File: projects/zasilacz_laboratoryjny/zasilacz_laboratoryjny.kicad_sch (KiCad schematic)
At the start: 99 parts, among them J1 OUT+, J10 PWRL−, J100 BARREL JACK, J101 BANANA JACK, J102 BANANA JACK, J103 OFF_BOARD, J104 OFF_BOARD, J105 OFF_BOARD, J106 OFF_BOARD, J107 OFF_BOARD, J108 OFF_BOARD, J109 OFF_BOARD, J11 VSET1, J110 OFF_BOARD, J111 OFF_BOARD, J112 OFF_BOARD, J113 OFF_BOARD, J114 OFF_BOARD, J115 OFF_BOARD, J116 OFF_BOARD, J117 OFF_BOARD, J118 OFF_BOARD, J119 OFF_BOARD, J12 VSET2, J120 OFF_BOARD, J121 OFF_BOARD, J122 OFF_BOARD, J13 OCPL+, J14 OCPL−, J15 VDOL+, J16 VDOL−, J17 OCP1, J18 OCP2, J19 OCP3, J2 OUT-, J20 OCP4, J21 OCP5, J22 OCP6, J23 OCP7, J24 OCP8, J3 PWRIN, J4 PWRSW, J5 VMPROBE, J6 VMPWR, J7 VMGND, J8 OCP0, J9 PWRL+, M1 DIGITAL_VM, P1 10kΩ, SW1 SW_SP8T, SW2 SW_SPST, T1 BC557, T2 BC557, T3 BC547, T4 BC547, T5 BC557, T6 BC557, T7 BC517, T8 BC547, U1 DB207, U2 LM317, Y1 3V

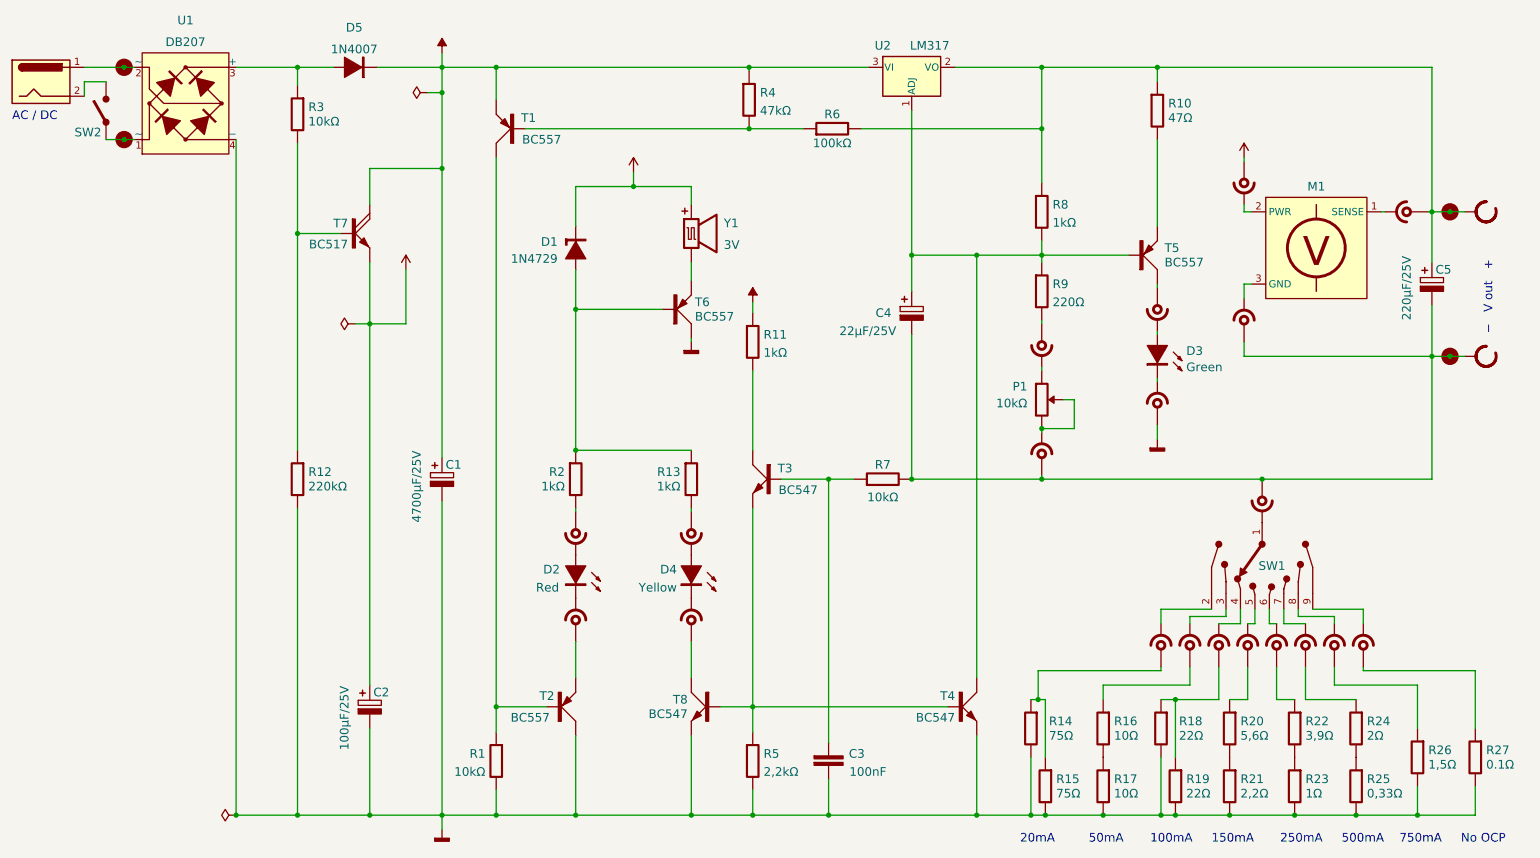
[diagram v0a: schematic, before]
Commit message: Zasilacz laboratoryjny - koniec
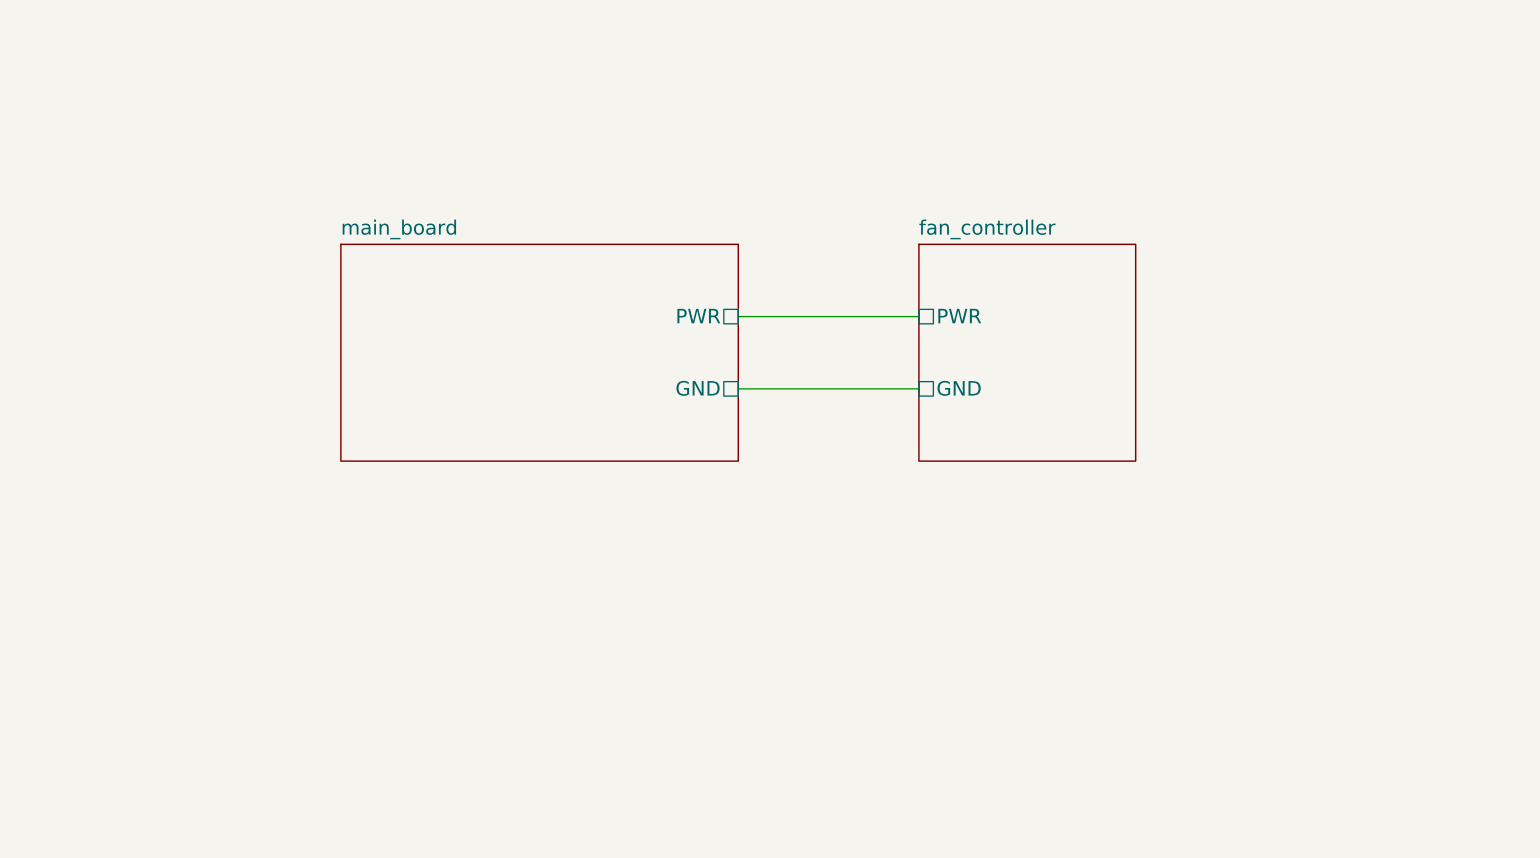
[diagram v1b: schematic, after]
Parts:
- removed C1: 4700μF/25V, VeeCad:RA3_6, symbol *Custom_Generic:C_Polarized
- removed C2: 100μF/25V, VeeCad:RA1_2, symbol *Custom_Generic:C_Polarized
- removed C3: 100nF, VeeCad:AX1_1N, symbol *Custom_Generic:C
- removed C4: 22μF/25V, VeeCad:RA1_2, symbol *Custom_Generic:C_Polarized
- removed C5: 220μF/25V, VeeCad:RA1_3, symbol *Custom_Generic:C_Polarized
- removed D1: 1N4729, VeeCad:AX2_1, symbol *Custom_Generic:D_zener
- removed D2: Red, symbol *Custom_Generic:LED
- removed D3: Green, symbol *Custom_Generic:LED
- removed D4: Yellow, symbol *Custom_Generic:LED
- removed D5: 1N4007, VeeCad:VERTAX_1U, symbol *Custom_Generic:D
- removed J1: OUT+, VeeCad:WIREPOINT, symbol *Custom_Generic:Wire_Solderpoint
- removed J10: PWRL−, VeeCad:SIP1, symbol *Custom_Generic:Conn_Point_M
- removed J100: BARREL JACK, symbol Connector:Barrel_Jack
- removed J101, J102: BANANA JACK, symbol *Custom_Generic:Conn_Jack
- removed J103, J104, J105, J106, J107, J108, J109, J110, J111, J112, J113, J114, J115, J116, J117, J118, J119, J120, J121, J122: OFF_BOARD, symbol *Custom_Generic:Conn_Point_F
- removed J11: VSET1, VeeCad:SIP1, symbol *Custom_Generic:Conn_Point_M
- removed J12: VSET2, VeeCad:SIP1, symbol *Custom_Generic:Conn_Point_M
- removed J13: OCPL+, VeeCad:SIP1, symbol *Custom_Generic:Conn_Point_M
- removed J14: OCPL−, VeeCad:SIP1, symbol *Custom_Generic:Conn_Point_M
- removed J15: VDOL+, VeeCad:SIP1, symbol *Custom_Generic:Conn_Point_M
- removed J16: VDOL−, VeeCad:SIP1, symbol *Custom_Generic:Conn_Point_M
- removed J17: OCP1, VeeCad:SIP1, symbol *Custom_Generic:Conn_Point_M
- removed J18: OCP2, VeeCad:SIP1, symbol *Custom_Generic:Conn_Point_M
- removed J19: OCP3, VeeCad:SIP1, symbol *Custom_Generic:Conn_Point_M
- removed J2: OUT-, VeeCad:WIREPOINT, symbol *Custom_Generic:Wire_Solderpoint
- removed J20: OCP4, VeeCad:SIP1, symbol *Custom_Generic:Conn_Point_M
- removed J21: OCP5, VeeCad:SIP1, symbol *Custom_Generic:Conn_Point_M
- removed J22: OCP6, VeeCad:SIP1, symbol *Custom_Generic:Conn_Point_M
- removed J23: OCP7, VeeCad:SIP1, symbol *Custom_Generic:Conn_Point_M
- removed J24: OCP8, VeeCad:SIP1, symbol *Custom_Generic:Conn_Point_M
- removed J3: PWRIN, VeeCad:WIREPOINT, symbol *Custom_Generic:Wire_Solderpoint
- removed J4: PWRSW, VeeCad:WIREPOINT, symbol *Custom_Generic:Wire_Solderpoint
- removed J5: VMPROBE, VeeCad:SIP1, symbol *Custom_Generic:Conn_Point_M
- removed J6: VMPWR, VeeCad:SIP1, symbol *Custom_Generic:Conn_Point_M
- removed J7: VMGND, VeeCad:SIP1, symbol *Custom_Generic:Conn_Point_M
- removed J8: OCP0, VeeCad:SIP1, symbol *Custom_Generic:Conn_Point_M
- removed J9: PWRL+, VeeCad:SIP1, symbol *Custom_Generic:Conn_Point_M
- removed M1: DIGITAL_VM, symbol *Custom_Generic:VM_DIGITAL
- removed P1: 10kΩ, symbol *Custom_Generic:P
- removed R1, R3, R7: 10kΩ, VeeCad:AX3_1N, symbol *Custom_Generic:R
- removed R10: 47Ω, VeeCad:VERTAX_2N, symbol *Custom_Generic:R
- removed R11: 1kΩ, VeeCad:AX3_1N, symbol *Custom_Generic:R
- removed R12: 220kΩ, VeeCad:AX3_1N, symbol *Custom_Generic:R
- removed R13: 1kΩ, VeeCad:VERTAX_2N_180, symbol *Custom_Generic:R
- removed R14, R15: 75Ω, VeeCad:AX3_1N, symbol *Custom_Generic:R
- removed R16, R17: 10Ω, VeeCad:VERTAX_1N, symbol *Custom_Generic:R
- removed R18, R19: 22Ω, VeeCad:AX3_1N, symbol *Custom_Generic:R
- removed R2: 1kΩ, VeeCad:VERTAX_1N_180, symbol *Custom_Generic:R
- removed R20: 5,6Ω, VeeCad:VERTAX_1N, symbol *Custom_Generic:R
- removed R21: 2,2Ω, VeeCad:VERTAX_1N, symbol *Custom_Generic:R
- removed R22: 3,9Ω, VeeCad:VERTAX2_1N, symbol *Custom_Generic:R
- removed R23: 1Ω, VeeCad:VERTAX2_1N, symbol *Custom_Generic:R
- removed R24: 2Ω, VeeCad:VERTAX2_1N, symbol *Custom_Generic:R
- removed R25: 0,33Ω, VeeCad:VERTAX2_1N, symbol *Custom_Generic:R
- removed R26: 1,5Ω, VeeCad:VERTAX2_1N, symbol *Custom_Generic:R
- removed R27: 0.1Ω, VeeCad:VERTAX2_1N, symbol *Custom_Generic:R
- removed R4: 47kΩ, VeeCad:AX3_1N, symbol *Custom_Generic:R
- removed R5: 2,2kΩ, VeeCad:AX3_1N, symbol *Custom_Generic:R
- removed R6: 100kΩ, VeeCad:AX3_1N, symbol *Custom_Generic:R
- removed R8: 1kΩ, VeeCad:VERTAX_1N, symbol *Custom_Generic:R
- removed R9: 220Ω, VeeCad:VERTAX_2N, symbol *Custom_Generic:R
- removed SW1: SW_SP8T, symbol *Custom_Generic:SW_SP8T
- removed SW2: SW_SPST, symbol *Custom_Generic:SW_SPST
- removed T1, T2, T6: BC557, VeeCad:TO92, symbol *Custom_Generic:PNP_BJT_CBE
- removed T3, T4, T8: BC547, VeeCad:TO92, symbol *Custom_Generic:NPN_BJT_CBE
- removed T5: BC557, VeeCad:TO92_ALT2, symbol *Custom_Generic:PNP_BJT_CBE
- removed T7: BC517, VeeCad:TO92, symbol *Custom_Generic:NPN_Darlington_EBC
- removed U1: DB207, VeeCad:DIP4_DB, symbol Custom_Generic:D_bridge_DIP
- removed U2: LM317, VeeCad:TO220, symbol Regulator_Linear:LM317_TO-220
- removed Y1: 3V, VeeCad:BUZR_12, symbol *Custom_Generic:Buzzer_Magnetic_Active
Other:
- added sheet fan_controller (fan_controller.kicad_sch)
- added sheet main_board (main_board.kicad_sch)
- note removed: "100mA"
- note removed: "150mA"
- note removed: "20mA"
- note removed: "250mA"
- note removed: "500mA"
- note removed: "50mA"
- note removed: "750mA"
- note removed: "AC / DC"
- note removed: "No OCP"
- note removed: "− V out +"
